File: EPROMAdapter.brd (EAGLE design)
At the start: 160 x 100 mm, 2 parts

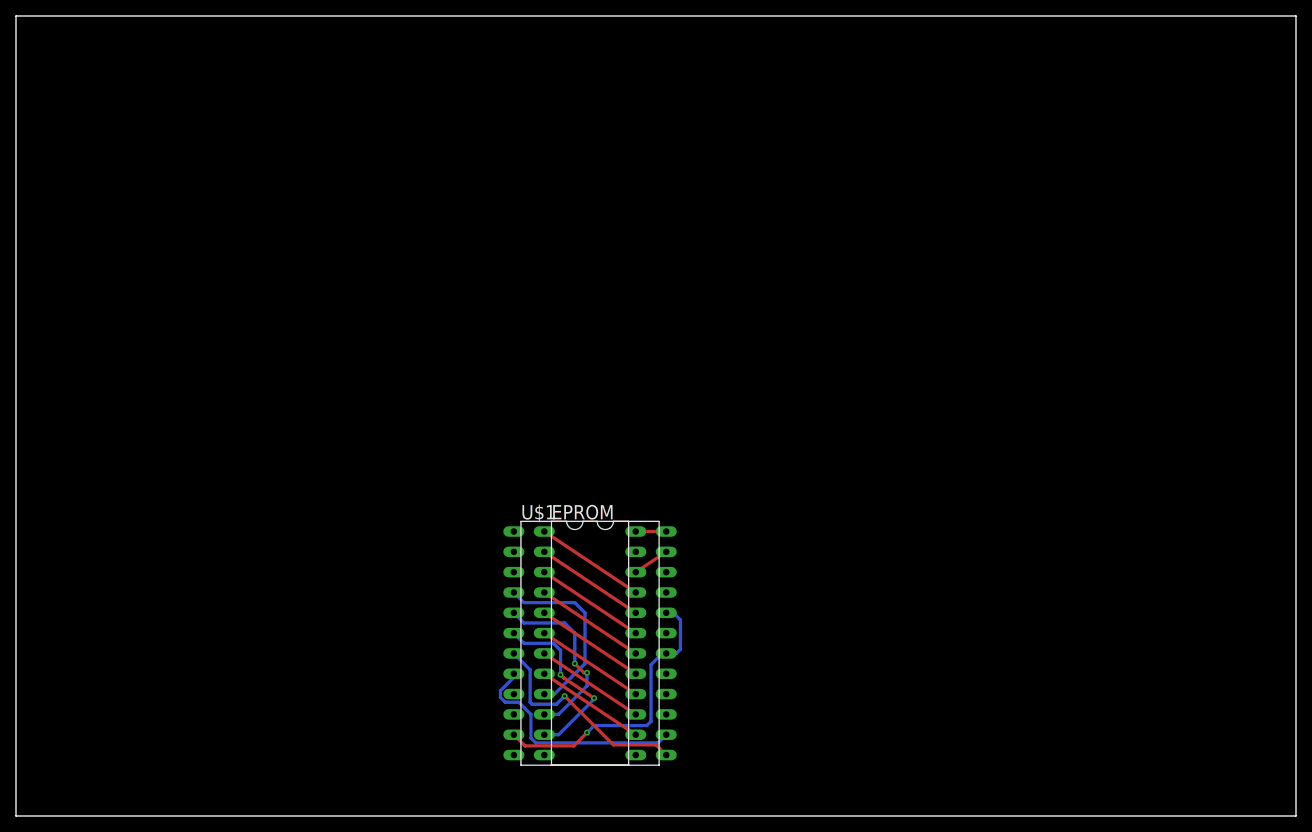
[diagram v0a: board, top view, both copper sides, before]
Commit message: wrapped that up
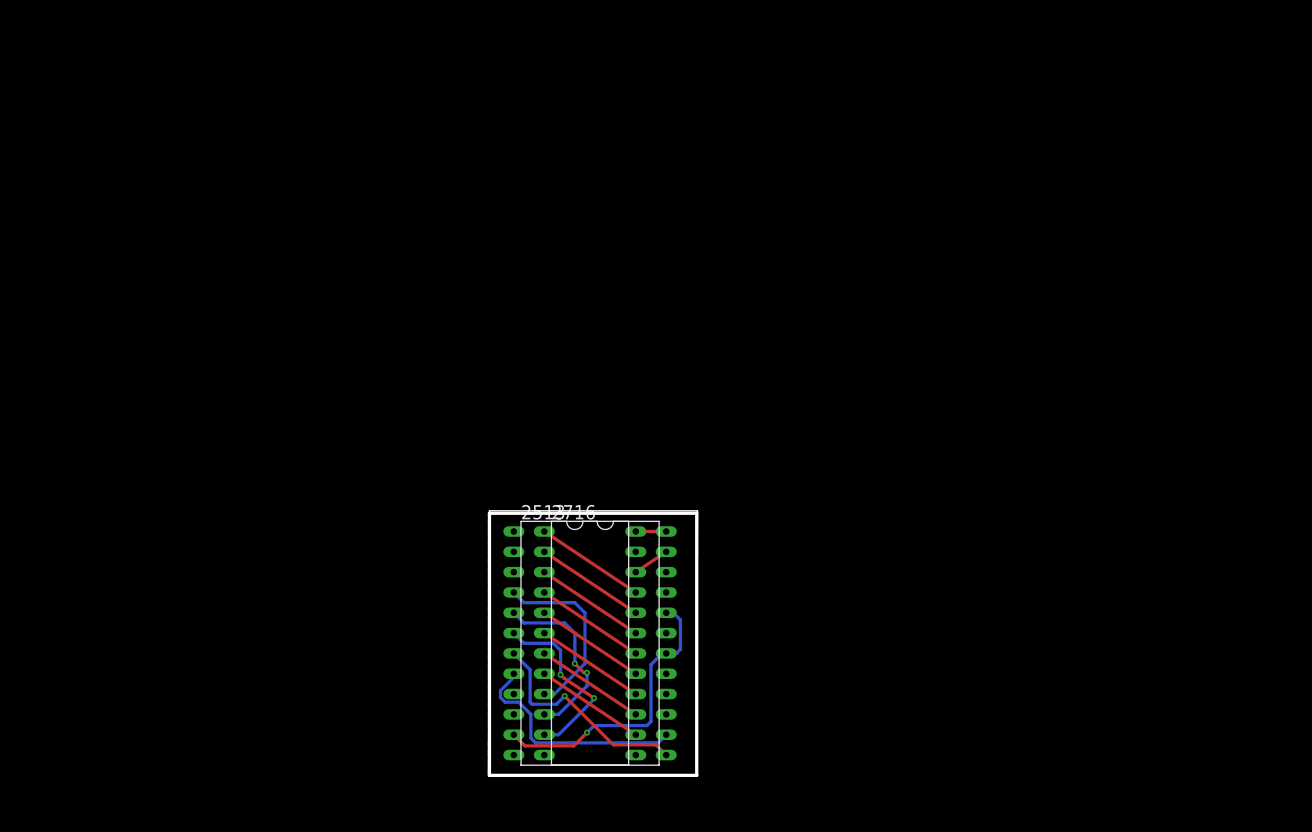
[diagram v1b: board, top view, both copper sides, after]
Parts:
- renumbered EPROM to 2716, U$1 to 2513
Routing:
- added copper zone on layer 1, net GND
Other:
- board size 160 x 100 mm -> 26.1 x 33.1 mm
- board text added: "2513 Character Gen. to 2716 EPROM Adapter"
- board text added: "github.com/bbenchoff/2513CharGenAdapter"
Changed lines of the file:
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@@
 <layer number="44" name="Drills" color="7" fill="1" visible="no" active="yes"/>
 <layer number="45" name="Holes" color="7" fill="1" visible="no" active="yes"/>
-<layer number="46" name="Milling" color="3" fill="1" visible="no" active="yes"/>
+<layer number="46" name="Milling" color="3" fill="1" visible="yes" active="yes"/>
 <layer number="47" name="Measures" color="7" fill="1" visible="no" active="yes"/>
 <layer number="48" name="Document" color="7" fill="1" visible="yes" active="yes"/>
@@
 <board>
 <plain>
-<wire x1="0" y1="0" x2="160" y2="0" width="0" layer="20"/>
-<wire x1="160" y1="0" x2="160" y2="100" width="0" layer="20"/>
-<wire x1="160" y1="100" x2="0" y2="100" width="0" layer="20"/>
-<wire x1="0" y1="100" x2="0" y2="0" width="0" layer="20"/>
-<text x="73.66" y="34.29" size="1.778" layer="22" font="vector" ratio="20" rot="MR270">Bottom towards board</text>
+<wire x1="59.055" y1="5.08" x2="85.07" y2="5.08" width="0" layer="20"/>
+<wire x1="85.07" y1="5.08" x2="85.197" y2="38.151" width="0" layer="20"/>
+<wire x1="85.197" y1="38.151" x2="59.182" y2="38.151" width="0" layer="20"/>
+<wire x1="59.182" y1="38.151" x2="59.055" y2="5.08" width="0" layer="20"/>
+<text x="75.819" y="34.29" size="1.778" layer="22" font="vector" ratio="20" rot="MR270">Bottom towards board</text>
+<text x="72.644" y="7.493" size="1.778" layer="27" font="vector" ratio="20" rot="R90">2513 Character Gen.
+to 2716 EPROM Adapter</text>
+<text x="83.82" y="33.02" size="0.8128" layer="27" font="vector" ratio="14" rot="R270">github.com/bbenchoff/2513CharGenAdapter</text>
+<wire x1="59.182" y1="37.846" x2="85.09" y2="37.846" width="0.4064" layer="46"/>
+<wire x1="85.09" y1="37.846" x2="85.09" y2="5.08" width="0.4064" layer="46"/>
+<wire x1="85.09" y1="5.08" x2="59.182" y2="5.08" width="0.4064" layer="46"/>
+<wire x1="59.182" y1="5.08" x2="59.182" y2="37.846" width="0.4064" layer="46"/>
 </plain>
 <attributes>
@@
 </autorouter>
 <elements>
-<element name="EPROM" library="memory" library_urn="urn:adsk.eagle:library:279" package="DIL24" package3d_urn="urn:adsk.eagle:package:19955/2" value="" x="73.66" y="21.59" smashed="yes" rot="R270">
+<element name="2716" library="memory" library_urn="urn:adsk.eagle:library:279" package="DIL24" package3d_urn="urn:adsk.eagle:package:19955/2" value="" x="73.66" y="21.59" smashed="yes" rot="R270">
 <attribute name="NAME" x="66.929" y="37.084" size="1.778" layer="25" ratio="10"/>
 <attribute name="VALUE" x="72.771" y="32.893" size="1.778" layer="27" ratio="10" rot="R270"/>
 </element>
-<element name="U$1" library="memory" package="DIL24" package3d_urn="urn:adsk.eagle:package:19955/2" value="2513-CHARACTER" x="69.85" y="21.59" smashed="yes" rot="R270">
+<element name="2513" library="memory" package="DIL24" package3d_urn="urn:adsk.eagle:package:19955/2" value="2513-CHARACTER" x="69.85" y="21.59" smashed="yes" rot="R270">
 <attribute name="NAME" x="63.119" y="37.084" size="1.778" layer="25" ratio="10"/>
 </element>
@@
 <signals>
 <signal name="VCC">
-<contactref element="U$1" pad="24"/>
-<contactref element="EPROM" pad="24"/>
+<contactref element="2513" pad="24"/>
+<contactref element="2716" pad="24"/>
 <wire x1="77.47" y1="35.56" x2="81.28" y2="35.56" width="0.4064" layer="1"/>
 </signal>
 <signal name="GND">
-<contactref element="U$1" pad="10"/>
-<contactref element="EPROM" pad="12"/>
-<contactref element="EPROM" pad="22"/>
-<contactref element="EPROM" pad="19"/>
-<wire x1="81.28" y1="22.86" x2="81.28" y2="30.48" width="0" layer="19" extent="1-1"/>
-<wire x1="62.23" y1="12.7" x2="81.28" y2="22.86" width="0" layer="19" extent="1-1"/>
-<wire x1="66.04" y1="7.62" x2="81.28" y2="22.86" width="0" layer="19" extent="1-1"/>
+<contactref element="2513" pad="10"/>
+<contactref element="2716" pad="12"/>
+<contactref element="2716" pad="22"/>
+<contactref element="2716" pad="19"/>
+<polygon width="0.4064" layer="1">
+<vertex x="59.055" y="37.719"/>
+<vertex x="85.09" y="37.719"/>
+<vertex x="85.09" y="5.08"/>
+<vertex x="59.055" y="5.08"/>
+</polygon>
 </signal>
 <signal name="A8">
-<contactref element="U$1" pad="22"/>
-<contactref element="EPROM" pad="23"/>
+<contactref element="2513" pad="22"/>
+<contactref element="2716" pad="23"/>
 <wire x1="81.28" y1="33.02" x2="77.47" y2="30.48" width="0.4064" layer="1"/>
 </signal>
 <signal name="A7">
-<contactref element="U$1" pad="21"/>
-<contactref element="EPROM" pad="1"/>
+<contactref element="2513" pad="21"/>
+<contactref element="2716" pad="1"/>
 <wire x1="66.04" y1="35.56" x2="77.47" y2="27.94" width="0.4064" layer="1"/>
 </signal>
 <signal name="A6">
-<contactref element="U$1" pad="20"/>
-<contactref element="EPROM" pad="2"/>
+<contactref element="2513" pad="20"/>
+<contactref element="2716" pad="2"/>
 <wire x1="66.04" y1="33.02" x2="77.47" y2="25.4" width="0.4064" layer="1"/>
 </signal>
 <signal name="A5">
-<contactref element="U$1" pad="19"/>
-<contactref element="EPROM" pad="3"/>
+<contactref element="2513" pad="19"/>
+<contactref element="2716" pad="3"/>
 <wire x1="66.04" y1="30.48" x2="77.47" y2="22.86" width="0.4064" layer="1"/>
 </signal>
 <signal name="A4">
-<contactref element="U$1" pad="18"/>
-<contactref element="EPROM" pad="4"/>
+<contactref element="2513" pad="18"/>
+<contactref element="2716" pad="4"/>
 <wire x1="66.04" y1="27.94" x2="77.47" y2="20.32" width="0.4064" layer="1"/>
 </signal>
 <signal name="A3">
-<contactref element="U$1" pad="17"/>
-<contactref element="EPROM" pad="5"/>
+<contactref element="2513" pad="17"/>
+<contactref element="2716" pad="5"/>
 <wire x1="66.04" y1="25.4" x2="77.47" y2="17.78" width="0.4064" layer="1"/>
 </signal>
 <signal name="A2">
-<contactref element="U$1" pad="16"/>
-<contactref element="EPROM" pad="6"/>
+<contactref element="2513" pad="16"/>
+<contactref element="2716" pad="6"/>
 <wire x1="66.04" y1="22.86" x2="77.47" y2="15.24" width="0.4064" layer="1"/>
 </signal>
 <signal name="A1">
-<contactref element="U$1" pad="15"/>
-<contactref element="EPROM" pad="7"/>
+<contactref element="2513" pad="15"/>
+<contactref element="2716" pad="7"/>
 <wire x1="66.04" y1="20.32" x2="77.47" y2="12.7" width="0.4064" layer="1"/>
 </signal>
 <signal name="A0">
-<contactref element="U$1" pad="14"/>
-<contactref element="EPROM" pad="8"/>
+<contactref element="2513" pad="14"/>
+<contactref element="2716" pad="8"/>
 <wire x1="66.04" y1="17.78" x2="77.47" y2="10.16" width="0.4064" layer="1"/>
 </signal>
 <signal name="D1">
-<contactref element="U$1" pad="4"/>
-<contactref element="EPROM" pad="9"/>
+<contactref element="2513" pad="4"/>
+<contactref element="2716" pad="9"/>
 <wire x1="66.04" y1="15.24" x2="67.31" y2="15.24" width="0.4064" layer="16"/>
 <wire x1="71.12" y1="19.05" x2="71.12" y2="25.4" width="0.4064" layer="16"/>
@@
 </signal>
 <signal name="D2">
-<contactref element="U$1" pad="5"/>
-<contactref element="EPROM" pad="10"/>
+<contactref element="2513" pad="5"/>
+<contactref element="2716" pad="10"/>
 <wire x1="62.23" y1="25.4" x2="63.5" y2="24.13" width="0.4064" layer="16"/>
 <wire x1="63.5" y1="24.13" x2="68.58" y2="24.13" width="0.4064" layer="16"/>
@@
 </signal>
 <signal name="D3">
-<contactref element="U$1" pad="6"/>
-<contactref element="EPROM" pad="11"/>
+<contactref element="2513" pad="6"/>
+<contactref element="2716" pad="11"/>
 <wire x1="66.04" y1="10.16" x2="67.818" y2="10.16" width="0.4064" layer="16"/>
 <wire x1="67.818" y1="10.16" x2="72.263" y2="14.605" width="0.4064" layer="16"/>
@@
 </signal>
 <signal name="D4">
-<contactref element="U$1" pad="7"/>
-<contactref element="EPROM" pad="13"/>
+<contactref element="2513" pad="7"/>
+<contactref element="2716" pad="13"/>
 <wire x1="62.23" y1="20.32" x2="64.262" y2="18.288" width="0.4064" layer="16"/>
 <wire x1="64.262" y1="18.288" x2="64.262" y2="14.224" width="0.4064" layer="16"/>
@@
 </signal>
 <signal name="D5">
-<contactref element="U$1" pad="8"/>
-<contactref element="EPROM" pad="14"/>
+<contactref element="2513" pad="8"/>
+<contactref element="2716" pad="14"/>
 <wire x1="81.28" y1="10.16" x2="80.264" y2="9.144" width="0.4064" layer="16"/>
 <wire x1="64.95875625" y1="9.144" x2="64.3636" y2="9.73915625" width="0.4064" layer="16"/>
@@
 </signal>
 <signal name="!CE">
-<contactref element="EPROM" pad="18"/>
-<contactref element="EPROM" pad="20"/>
-<contactref element="U$1" pad="11"/>
+<contactref element="2716" pad="18"/>
+<contactref element="2716" pad="20"/>
+<contactref element="2513" pad="11"/>
 <wire x1="62.23" y1="10.16" x2="63.627" y2="8.763" width="0.4064" layer="1"/>
 <wire x1="69.723" y1="8.763" x2="71.374" y2="10.414" width="0.4064" layer="1"/>
@@
 </drawing>
 <compatibility>
+<note version="6.3" minversion="6.2.2" severity="warning">
+Since Version 6.2.2 text objects can contain more than one line,
+which will not be processed correctly with this version.
+</note>
 <note version="8.2" severity="warning">
 Since Version 8.2, EAGLE supports online libraries. The ids
